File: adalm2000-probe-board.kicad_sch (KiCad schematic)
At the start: 14 parts, among them J1 ADALM200 INPUT, J2 MODULE OUTPUT, J3 Ch1, J4 Ch2, J5 V+/W1, J6 V-/W2, SW1 SW_CH1_CPL, SW2 SW_CH1_GND_REF, SW3 SW_CH2_CPL, SW4 SW_CH2_GND_REF, SW5 SW_OUT_1, SW6 SW_OUT_2

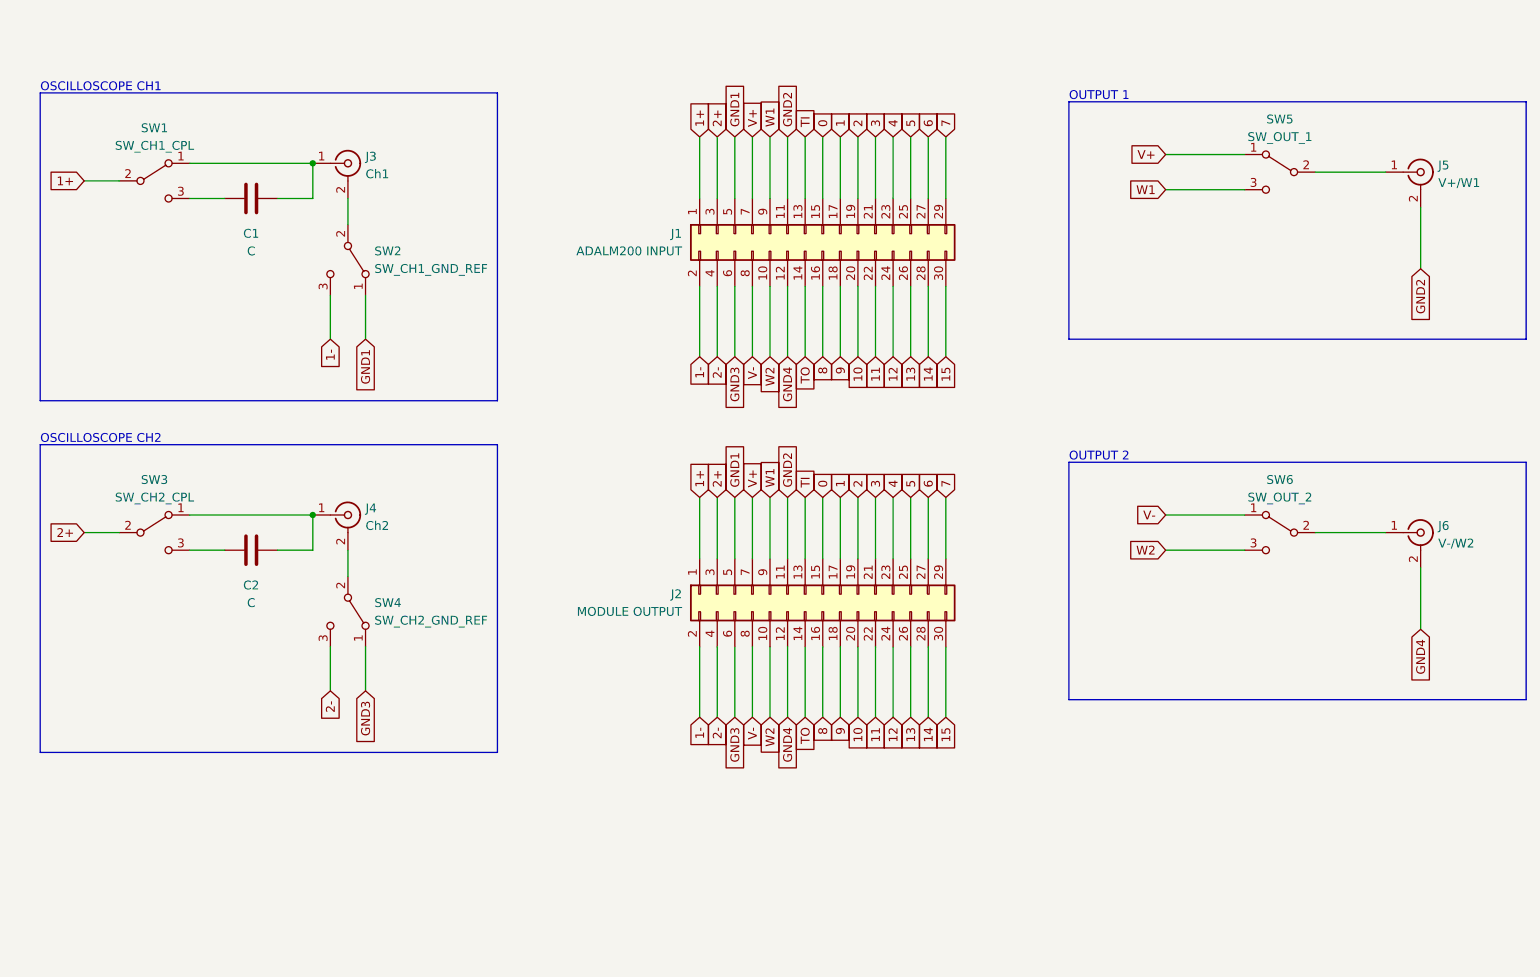
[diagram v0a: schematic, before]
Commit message: Initial PCB design
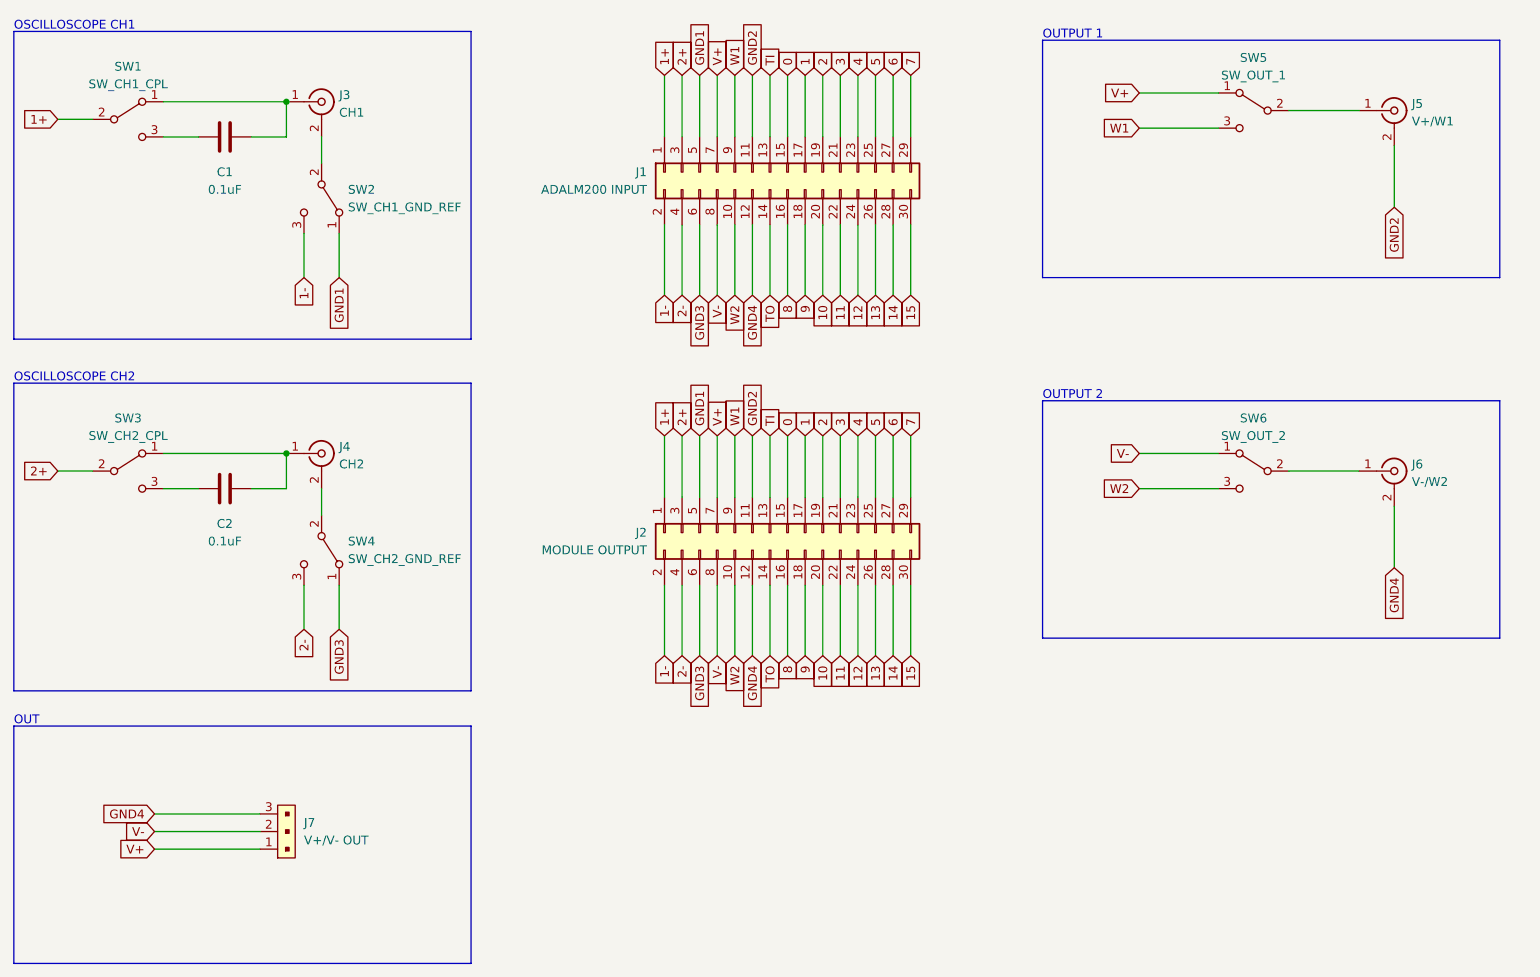
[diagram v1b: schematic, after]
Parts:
- added J7: V+/V- OUT, digikey-footprints:PinHeader_1x3_P2.54_Drill1.1mm, symbol dk_Rectangular-Connectors-Headers-Male-Pins:61300311121
- C1, C2: value C -> 0.1uF; footprint (none) -> Capacitor_SMD:C_0805_2012Metric
- J1: footprint Connector_IDC:IDC-Header_2x15_P2.54mm_Vertical -> Connector_IDC:IDC-Header_2x15_P2.54mm_Horizontal
- J2: footprint Connector_IDC:IDC-Header_2x15_P2.54mm_Vertical -> Jonnes Library:IDC-Header_2x15_P2.54mm_Horizontal - Pin 1 on left from front view
- J3: value Ch1 -> CH1; footprint (none) -> w_conn_rf:bnc_90_1-1337543-0
- J4: value Ch2 -> CH2; footprint (none) -> w_conn_rf:bnc_90_1-1337543-0
- J5, J6: footprint (none) -> w_conn_rf:bnc_90_1-1337543-0
- SW1, SW2, SW3, SW4, SW5, SW6: footprint (none) -> KiCad:SS12D00G3
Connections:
- net GND4: now also J7.3
- net V+: now also J7.1
- net V-: now also J7.2
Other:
- note added: "OUT"
- company: (none) -> Eng. Jonnes Nascimento
- title: (none) -> ADALM2000 Probe Board
- moved on the sheet: C1, C2, J1, J2, J3, J4, J5, J6, SW1, SW2, SW3, SW4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

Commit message: Initial PCB design
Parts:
- J1: footprint Connector_IDC:IDC-Header_2x15_P2.54mm_Horizontal -> Jonnes Library:PinSocket_2x15_P2.54mm_Horizontal
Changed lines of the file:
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@@
       (effects (font (size 1.27 1.27)) (justify left))
     )
-    (property "Footprint" "Connector_IDC:IDC-Header_2x15_P2.54mm_Horizontal" (id 2) (at 153.67 59.69 0)
+    (property "Footprint" "Jonnes Library:PinSocket_2x15_P2.54mm_Horizontal" (id 2) (at 153.67 59.69 0)
       (effects (font (size 1.27 1.27)) hide)
     )
@@
     )
     (path "/01e8a7f1-e668-442f-9994-925c867ee32b"
-      (reference "J1") (unit 1) (value "ADALM200 INPUT") (footprint "Connector_IDC:IDC-Header_2x15_P2.54mm_Horizontal")
+      (reference "J1") (unit 1) (value "ADALM200 INPUT") (footprint "Jonnes Library:PinSocket_2x15_P2.54mm_Horizontal")
     )
     (path "/d2fc562b-36d8-46a5-80f9-e350584d36cd"
